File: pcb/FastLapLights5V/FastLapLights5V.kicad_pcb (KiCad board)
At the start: 4 copper layers, 27.3 x 40 mm, 29 parts, among them IC1 74HCT1G125GV,125, J1 POWER_CON, J2 SWD, J3 I2C, J4 IO, U1 STM32C011F4Px, U2 AP63205WU, U3 AP2112K-3.3, U4 BD33FC0FP

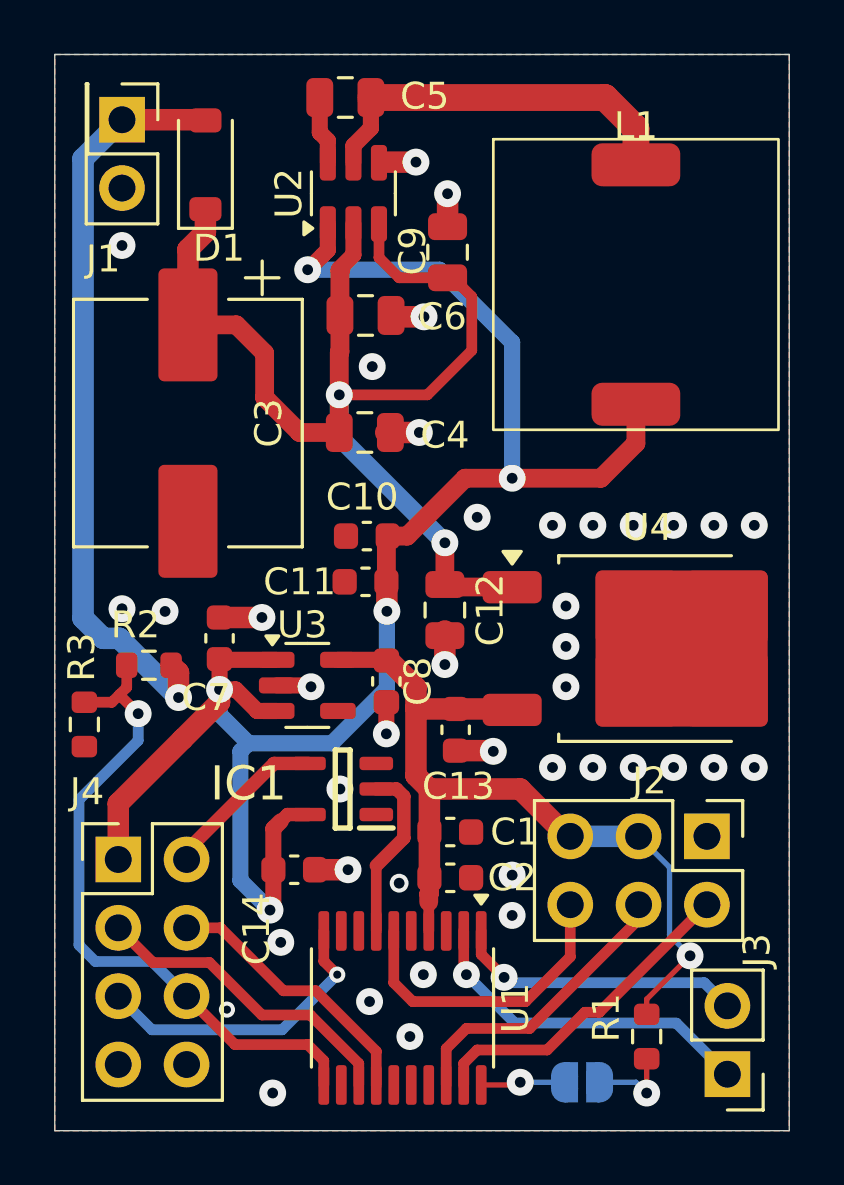
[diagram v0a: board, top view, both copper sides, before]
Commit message: change jlcpcb parts
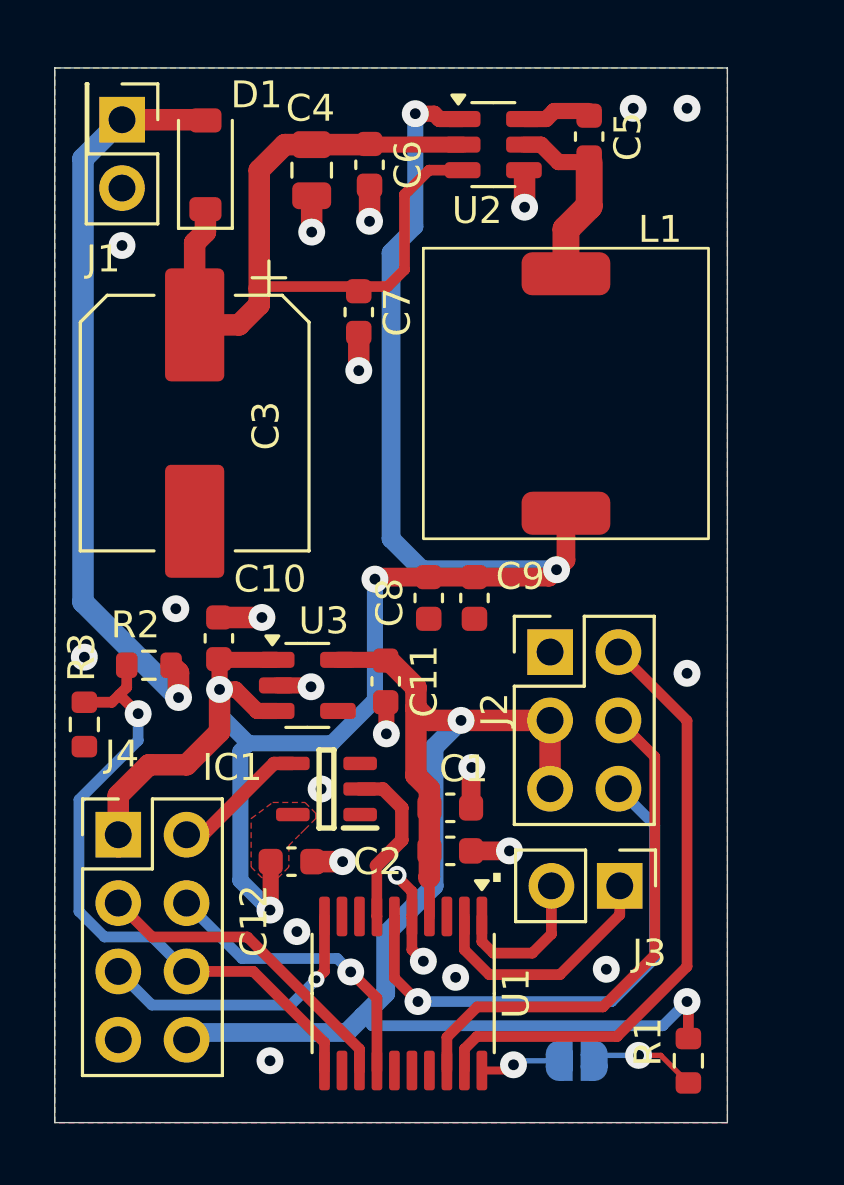
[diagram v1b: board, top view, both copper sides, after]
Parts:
- removed the C12 at (57.0, 107.3)
- removed C13: 22uF, Capacitor_SMD:C_0603_1608Metric
- removed the C7 at (48.6, 108.4)
- removed the C8 at (54.8, 110.0)
- removed U4: BD33FC0FP, Package_TO_SOT_SMD:TO-252-2
- added C10: 4.7uF, Capacitor_SMD:C_0603_1608Metric, F.Cu at (48.6, 108.4)
- added C11: 4.7uF, Capacitor_SMD:C_0603_1608Metric, F.Cu at (54.8, 110.0)
- C3: value 100uF -> 220uF; footprint Library:CP_Elec_A768KS227M1VLAE024 -> Library:CP_220_Honor_Elec_HV1E227M0810PZ
- C5: value 100nF -> 0.1uF; footprint Capacitor_SMD:C_0805_2012Metric -> Capacitor_SMD:C_0603_1608Metric
- C6: footprint Capacitor_SMD:C_0805_2012Metric -> Capacitor_SMD:C_0603_1608Metric
- C7: renamed from C9; footprint Capacitor_SMD:C_0805_2012Metric -> Capacitor_SMD:C_0603_1608Metric
- L1: value 22.8uH -> 22uH; footprint Library:L_EATON_DR1030-220-R -> Library:L_Chilisin_Elec_BPSC00101140220M00
- moved C4 9.95 mm to (52.0, 91.0), turned to -90 degrees
- moved C5 9.18 mm to (62.4, 89.8), turned to 90 degrees
- moved J2 9.00 mm to (60.9, 108.9), turned to 0 degrees
- moved J3 8.06 mm to (63.5, 117.6), turned to -90 degrees
- moved C6 5.60 mm to (54.2, 90.8), turned to -90 degrees
- moved U2 5.51 mm to (58.8, 90.0), turned to 0 degrees
- moved L1 4.81 mm to (61.5, 99.3)
- moved C9 4.09 mm to (58.1, 106.9), turned to -90 degrees
- moved C7 3.98 mm to (53.8, 96.3), turned to -90 degrees
- moved C8 3.25 mm to (56.4, 106.9), turned to -90 degrees
- moved R1 1.79 mm to (66.0, 124.1)
- moved C2 1.00 mm to (57.2, 116.3)
- moved J4 0.92 mm to (44.9, 115.7)
- moved C1 0.90 mm to (57.2, 114.7)
- moved JP1 0.82 mm to (61.9, 124.1)
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- renumbered C14 to C12, C10 to C8, C11 to C9
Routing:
- net +3.3V: track 32.8 -> 53.2 mm, vias 1 -> 2
- net /VRAIL_CAP: track 44.9 -> 31.1 mm, vias 2 -> 0
- net /SWD_SWCLK: track 12.3 -> 23.1 mm
- net /SWD_SWDIO: track 11.0 -> 19.5 mm
- net /SWD_NRST: track 11.4 -> 19.9 mm, vias 0 -> 1
- net Net-(U2-SW): track 14.4 -> 7.20 mm
- net /I2C_SCL: track 10.8 -> 5.78 mm, vias 1 -> 0
- net GND: track 12.9 -> 16.5 mm, vias 40 -> 23
- net /I2C_SDA: track 12.9 -> 9.39 mm, vias 1 -> 0
- net +5V: track 67.5 -> 68.7 mm
- net /START_LIGHTS_5V: track 6.22 -> 5.05 mm
- net /TRACK_LIGHTS_R: track 10.2 -> 11.2 mm, vias 0 -> 1
- net /IO_POWER_RAIL_DATA: track 25.2 -> 24.3 mm
- net Net-(JP1-A): track 3.19 -> 4.01 mm
- net /IO_POWER_RAIL_INT: track 11.3 -> 10.7 mm
- added copper zone on F.Cu, net +5V
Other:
- board size 27.3 x 40 mm -> 25 x 39.2 mm
- board text added: "."
